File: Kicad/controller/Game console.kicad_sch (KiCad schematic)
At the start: 31 parts, among them J1 Conn_01x04, J2 Conn_01x04, J3 Conn_01x02, J4 Conn_01x02, Q1 PN2222A, Q2 PN2222A, SW10 B, SW11 Menu, SW12 X, SW13 Y, SW14 View, SW3 D Pad top, SW4 D Pad right, SW5 D Pad Left, SW6 A, SW7 D Pad bottom, SW8 Reset, SW9 Home, U1 MCP3008

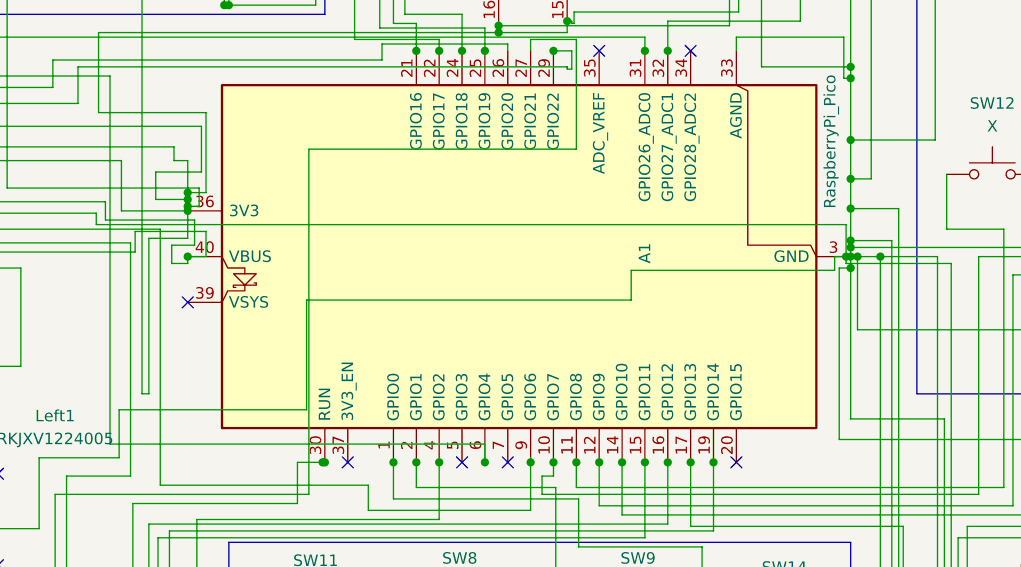
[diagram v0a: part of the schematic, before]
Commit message: doing the layout for pcb so I can make the perfect pcb board
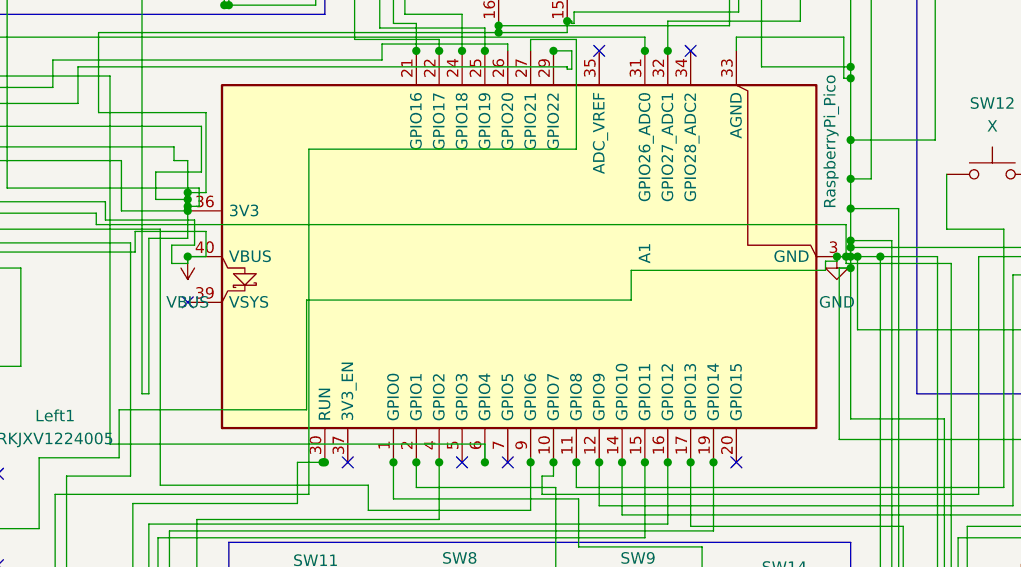
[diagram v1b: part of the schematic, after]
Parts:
- C3: footprint (none) -> Capacitor_THT:CP_Radial_D5.0mm_P2.00mm
- D2: footprint (none) -> LED_THT:LED_D3.0mm
- J3, J4: footprint (none) -> Connector_JST:JST_PH_B2B-PH-K_1x02_P2.00mm_Vertical
- R1, R2, R3: footprint (none) -> Resistor_THT:R_Axial_DIN0207_L6.3mm_D2.5mm_P10.16mm_Horizontal
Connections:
- net GND: now also D2.1 (K)
- net VBUS: now also A1.40 (VBUS), D1.1 (K), D3.1 (K), J3.1 (Pin_1), J4.1 (Pin_1)
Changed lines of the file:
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@@
 	)
 	(junction
+		(at 179.07 77.47)
+		(diameter 0)
+		(color 0 0 0 0)
+	)
+	(junction
 		(at 201.422 72.136)
 		(diameter 0)
@@
 	(wire
 		(pts
-			(xy 156.21 78.994) (xy 178.816 78.994)
-		)
-		(stroke
-			(width 0)
-			(type default)
-		)
-	)
-	(wire
-		(pts
 			(xy 149.86 51.562) (xy 149.606 51.562)
 		)
@@
 	(wire
 		(pts
+			(xy 179.07 77.47) (xy 179.832 77.47)
+		)
+		(stroke
+			(width 0)
+			(type default)
+		)
+	)
+	(wire
+		(pts
 			(xy 155.194 100.076) (xy 155.194 100.33)
 		)
@@
 	(wire
 		(pts
-			(xy 178.816 78.994) (xy 178.816 77.47)
-		)
-		(stroke
-			(width 0)
-			(type default)
-		)
-	)
-	(wire
-		(pts
 			(xy 215.9 66.548) (xy 203.2 66.548)
 		)
@@
 	(wire
 		(pts
-			(xy 178.816 77.47) (xy 179.832 77.47)
-		)
-		(stroke
-			(width 0)
-			(type default)
-		)
-	)
-	(wire
-		(pts
 			(xy 88.392 89.662) (xy 51.562 89.662)
 		)
@@
 	(wire
 		(pts
+			(xy 178.816 77.47) (xy 179.07 77.47)
+		)
+		(stroke
+			(width 0)
+			(type default)
+		)
+	)
+	(wire
+		(pts
 			(xy 93.472 101.854) (xy 93.472 114.808)
 		)
@@
 	(wire
 		(pts
+			(xy 177.8 77.978) (xy 179.07 77.978)
+		)
+		(stroke
+			(width 0)
+			(type default)
+		)
+	)
+	(wire
+		(pts
 			(xy 162.814 100.33) (xy 162.814 107.442)
 		)
@@
 	(wire
 		(pts
+			(xy 179.07 77.978) (xy 179.07 77.47)
+		)
+		(stroke
+			(width 0)
+			(type default)
+		)
+	)
+	(wire
+		(pts
 			(xy 128.27 36.068) (xy 128.27 52.07)
 		)
@@
 	(wire
 		(pts
+			(xy 156.21 78.994) (xy 177.8 78.994)
+		)
+		(stroke
+			(width 0)
+			(type default)
+		)
+	)
+	(wire
+		(pts
+			(xy 177.8 78.994) (xy 177.8 77.978)
+		)
+		(stroke
+			(width 0)
+			(type default)
+		)
+	)
+	(wire
+		(pts
 			(xy 129.794 100.33) (xy 129.794 104.394)
 		)
@@
 			)
 		)
-		(property "Footprint" ""
+		(property "Footprint" "Connector_JST:JST_PH_B2B-PH-K_1x02_P2.00mm_Vertical"
 			(at 35.814 99.822 0)
 			(hide yes)
@@
 	)
 	(symbol
+		(lib_id "power:GND")
+		(at 179.07 77.47 0)
+		(unit 1)
+		(body_style 1)
+		(exclude_from_sim no)
+		(in_bom yes)
+		(on_board yes)
+		(in_pos_files yes)
+		(dnp no)
+		(fields_autoplaced yes)
+		(property "Reference" "#PWR04"
+			(at 179.07 83.82 0)
+			(hide yes)
+			(show_name no)
+			(do_not_autoplace no)
+			(effects
+				(font
+					(size 1.27 1.27)
+				)
+			)
+		)
+		(property "Value" "GND"
+			(at 179.07 82.55 0)
+			(show_name no)
+			(do_not_autoplace no)
+			(effects
+				(font
+					(size 1.27 1.27)
+				)
+			)
+		)
+		(property "Footprint" ""
+			(at 179.07 77.47 0)
+			(hide yes)
+			(show_name no)
+			(do_not_autoplace no)
+			(effects
+				(font
+					(size 1.27 1.27)
+				)
+			)
+		)
+		(property "Datasheet" ""
+			(at 179.07 77.47 0)
+			(hide yes)
+			(show_name no)
+			(do_not_autoplace no)
+			(effects
+				(font
+					(size 1.27 1.27)
+				)
+			)
+		)
+		(property "Description" "Power symbol creates a global label with name \"GND\" , ground"
+			(at 179.07 77.47 0)
+			(hide yes)
+			(show_name no)
+			(do_not_autoplace no)
+			(effects
+				(font
+					(size 1.27 1.27)
+				)
+			)
+		)
+		(pin "1"
+		)
+		(instances
+			(project "Game console"
+				(path "/5d92d208-f11d-47b0-aded-0294da1c15f0"
+					(reference "#PWR04")
+					(unit 1)
+				)
+			)
+		)
+	)
+	(symbol
 		(lib_id "Switch:SW_Push")
 		(at 156.972 119.38 0)
@@
 			)
 		)
-		(property "Footprint" ""
+		(property "Footprint" "Capacitor_THT:CP_Radial_D5.0mm_P2.00mm"
 			(at 20.7772 107.95 0)
 			(hide yes)
@@
 			)
 		)
-		(property "Footprint" ""
+		(property "Footprint" "LED_THT:LED_D3.0mm"
 			(at 17.526 96.012 0)
 			(hide yes)
@@
 			)
 		)
-		(property "Footprint" ""
+		(property "Footprint" "Resistor_THT:R_Axial_DIN0207_L6.3mm_D2.5mm_P10.16mm_Horizontal"
 			(at 42.418 140.208 90)
 			(hide yes)
@@
 			)
 		)
-		(property "Footprint" ""
+		(property "Footprint" "Resistor_THT:R_Axial_DIN0207_L6.3mm_D2.5mm_P10.16mm_Horizontal"
 			(at 18.288 80.772 90)
 			(hide yes)
@@
 			)
 		)
-		(property "Footprint" ""
+		(property "Footprint" "Resistor_THT:R_Axial_DIN0207_L6.3mm_D2.5mm_P10.16mm_Horizontal"
 			(at 28.448 80.264 90)
 			(hide yes)
@@
 			)
 		)
-		(property "Footprint" ""
+		(property "Footprint" "Connector_JST:JST_PH_B2B-PH-K_1x02_P2.00mm_Vertical"
 			(at 19.558 127.508 0)
 			(hide yes)
@@
 					(unit 1)
 				)
+			)
+		)
+	)
+	(symbol
+		(lib_id "power:VBUS")
+		(at 106.934 77.47 180)
+		(unit 1)
+		(body_style 1)
+		(exclude_from_sim no)
+		(in_bom yes)
+		(on_board yes)
+		(in_pos_files yes)
+		(dnp no)
+		(fields_autoplaced yes)
+		(property "Reference" "#PWR03"
+			(at 106.934 73.66 0)
+			(hide yes)
+			(show_name no)
+			(do_not_autoplace no)
+			(effects
+				(font
+					(size 1.27 1.27)
+				)
+			)
+		)
+		(property "Value" "VBUS"
+			(at 106.934 82.55 0)
+			(show_name no)
+			(do_not_autoplace no)
+			(effects
+				(font
+					(size 1.27 1.27)
+				)
+			)
+		)
+		(property "Footprint" ""
+			(at 106.934 77.47 0)
+			(hide yes)
+			(show_name no)
+			(do_not_autoplace no)
+			(effects
+				(font
+					(size 1.27 1.27)
+				)
+			)
+		)
+		(property "Datasheet" ""
+			(at 106.934 77.47 0)
+			(hide yes)
+			(show_name no)
+			(do_not_autoplace no)
+			(effects
+				(font
+					(size 1.27 1.27)
+				)
+			)
+		)
+		(property "Description" "Power symbol creates a global label with name \"VBUS\""
+			(at 106.934 77.47 0)
+			(hide yes)
+			(show_name no)
+			(do_not_autoplace no)
+			(effects
+				(font
+					(size 1.27 1.27)
+				)
+			)
+		)
+		(pin "1"
+		)
+		(instances
+			(project "Game console"
+				(path "/5d92d208-f11d-47b0-aded-0294da1c15f0"
+					(reference "#PWR03")
+					(unit 1)
+				)
